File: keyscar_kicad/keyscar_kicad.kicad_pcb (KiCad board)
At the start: 2 copper layers, 21 x 26.8 mm, 28 parts, among them SW1 SSSS211603, SW2 SSSS211603, SW5_MASTER_EXEC1 TSA453G50-250, SW6_SLAVE_EXEC2 TSA453G50-250

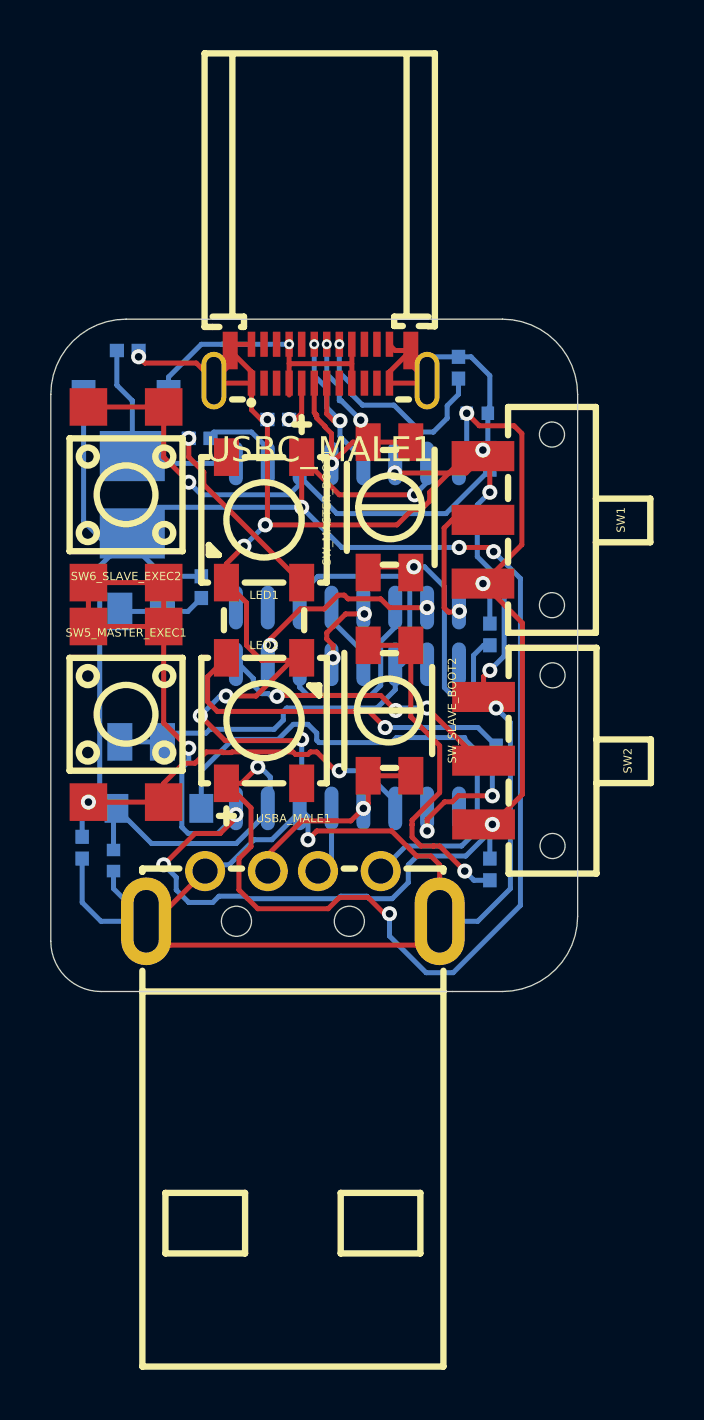
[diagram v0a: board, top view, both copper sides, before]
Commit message: yippee
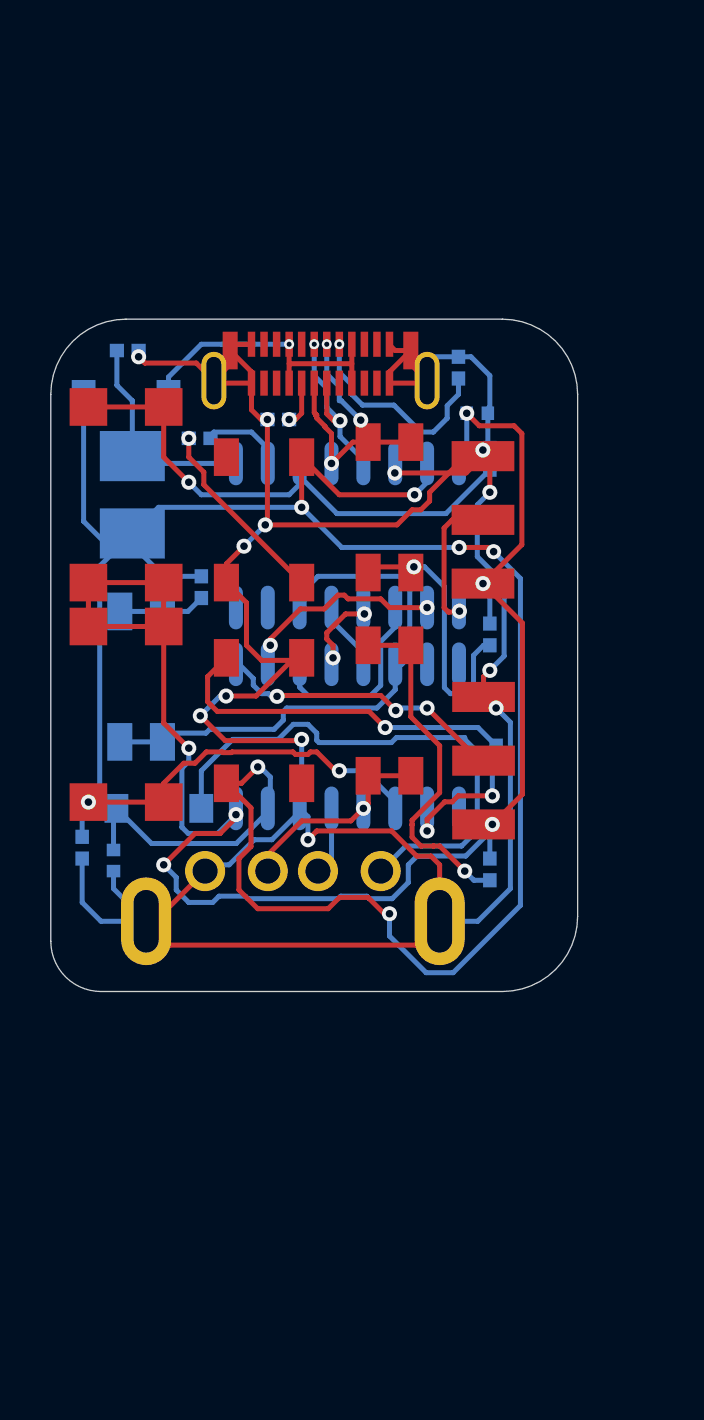
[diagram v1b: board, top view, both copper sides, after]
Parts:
- added G***: LOGO, Library:hack_logo, B.Cu at (264.4, 78.2)
- added G***: LOGO, Library:stasis_logo, B.Cu at (264.5, 93.0)
- added G***: LOGO, Library:hackclub_logo, B.Cu at (264.5, 85.2)
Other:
- board text added: "@Ninjago77"
- board text added: "Keyscar"
- board text added: "MASTER"
- board text added: "SLAVE"
